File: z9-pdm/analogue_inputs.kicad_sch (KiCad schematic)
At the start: 0 parts

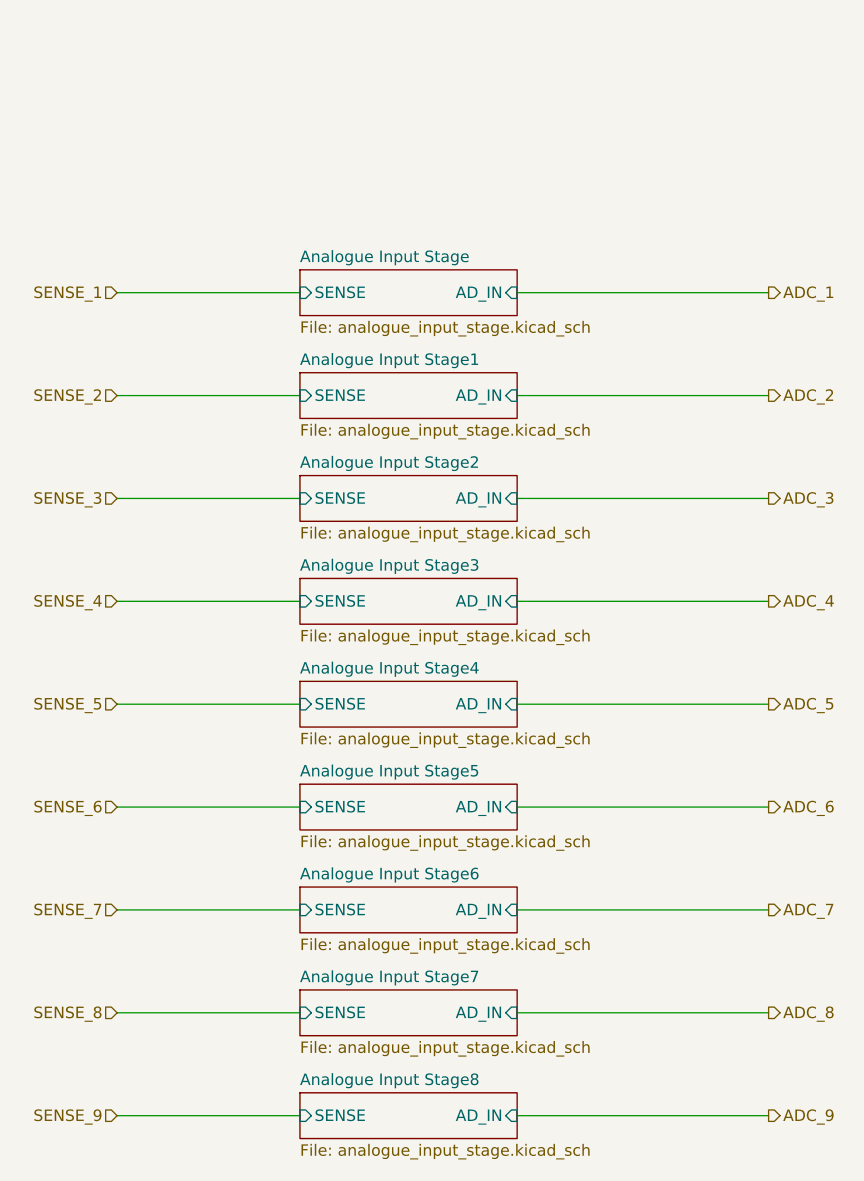
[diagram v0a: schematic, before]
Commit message: pre replicate analogue chans
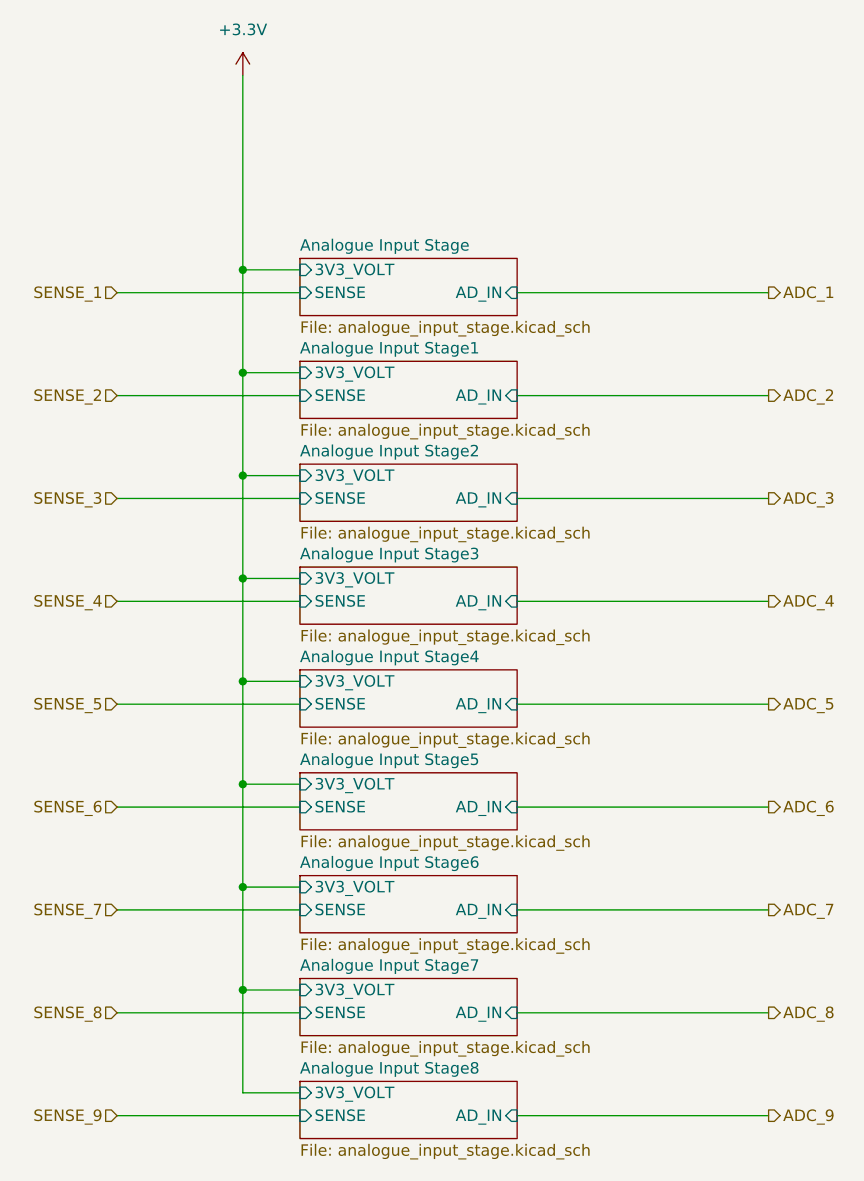
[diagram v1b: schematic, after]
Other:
- sheet Analogue Input Stage ports: added 3V3_VOLT; removed none
- sheet Analogue Input Stage1 ports: added 3V3_VOLT; removed none
- sheet Analogue Input Stage2 ports: added 3V3_VOLT; removed none
- sheet Analogue Input Stage3 ports: added 3V3_VOLT; removed none
- sheet Analogue Input Stage4 ports: added 3V3_VOLT; removed none
- sheet Analogue Input Stage5 ports: added 3V3_VOLT; removed none
- sheet Analogue Input Stage6 ports: added 3V3_VOLT; removed none
- sheet Analogue Input Stage7 ports: added 3V3_VOLT; removed none
- sheet Analogue Input Stage8 ports: added 3V3_VOLT; removed none

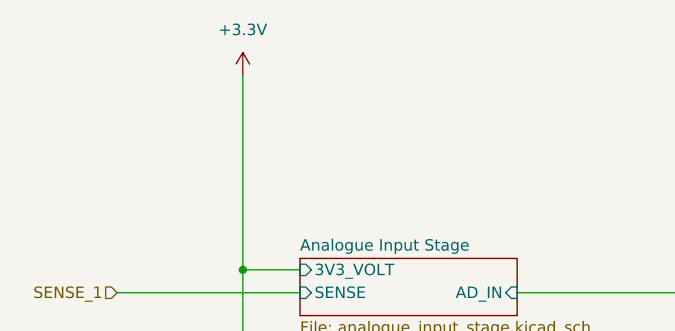
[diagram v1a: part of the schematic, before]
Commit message: x
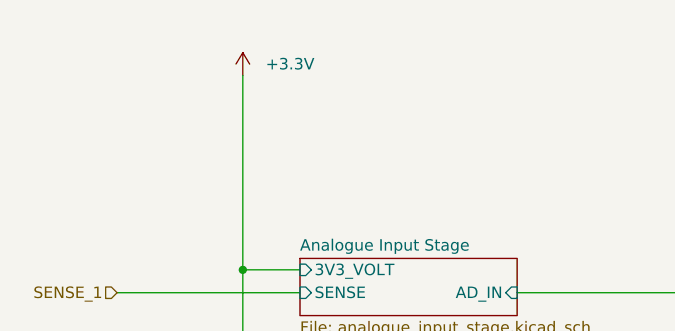
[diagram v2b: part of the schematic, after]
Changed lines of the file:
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@@
 		(dnp no)
 		(fields_autoplaced yes)
-		(property "Reference" "#PWR04901"
+		(property "Reference" "#PWR090"
 			(at 130.81 25.4 0)
 			(effects
@@
 		)
 		(property "Value" "+3.3V"
-			(at 130.81 16.51 0)
+			(at 133.35 20.3199 0)
 			(effects
 				(font
 					(size 1.27 1.27)
 				)
+				(justify left)
 			)
 		)
@@
 			(project ""
 				(path "/b643db5c-578e-4b48-aafc-cc4190db582a/4bf3a54e-2413-4742-bb3c-6ced251716e8"
-					(reference "#PWR04901")
+					(reference "#PWR090")
 					(unit 1)
 				)

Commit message: passes sch drc
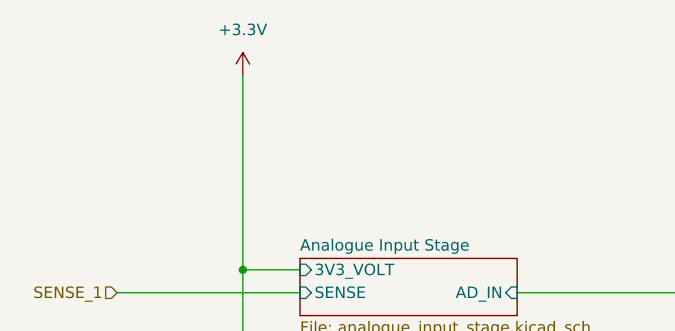
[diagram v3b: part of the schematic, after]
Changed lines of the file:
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@@
 		)
 		(property "Value" "+3.3V"
-			(at 133.35 20.3199 0)
+			(at 130.81 16.51 0)
 			(effects
 				(font
 					(size 1.27 1.27)
 				)
-				(justify left)
 			)
 		)
